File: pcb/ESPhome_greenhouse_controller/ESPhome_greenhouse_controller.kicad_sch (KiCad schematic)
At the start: 10 parts, among them K1 SANYOU_SRD_Form_C, K2 SANYOU_SRD_Form_C, K3 SANYOU_SRD_Form_C, K4 SANYOU_SRD_Form_C, K5 SANYOU_SRD_Form_C, K6 SANYOU_SRD_Form_C, U1 PC817, U2 PC817, U3 INA219AxD

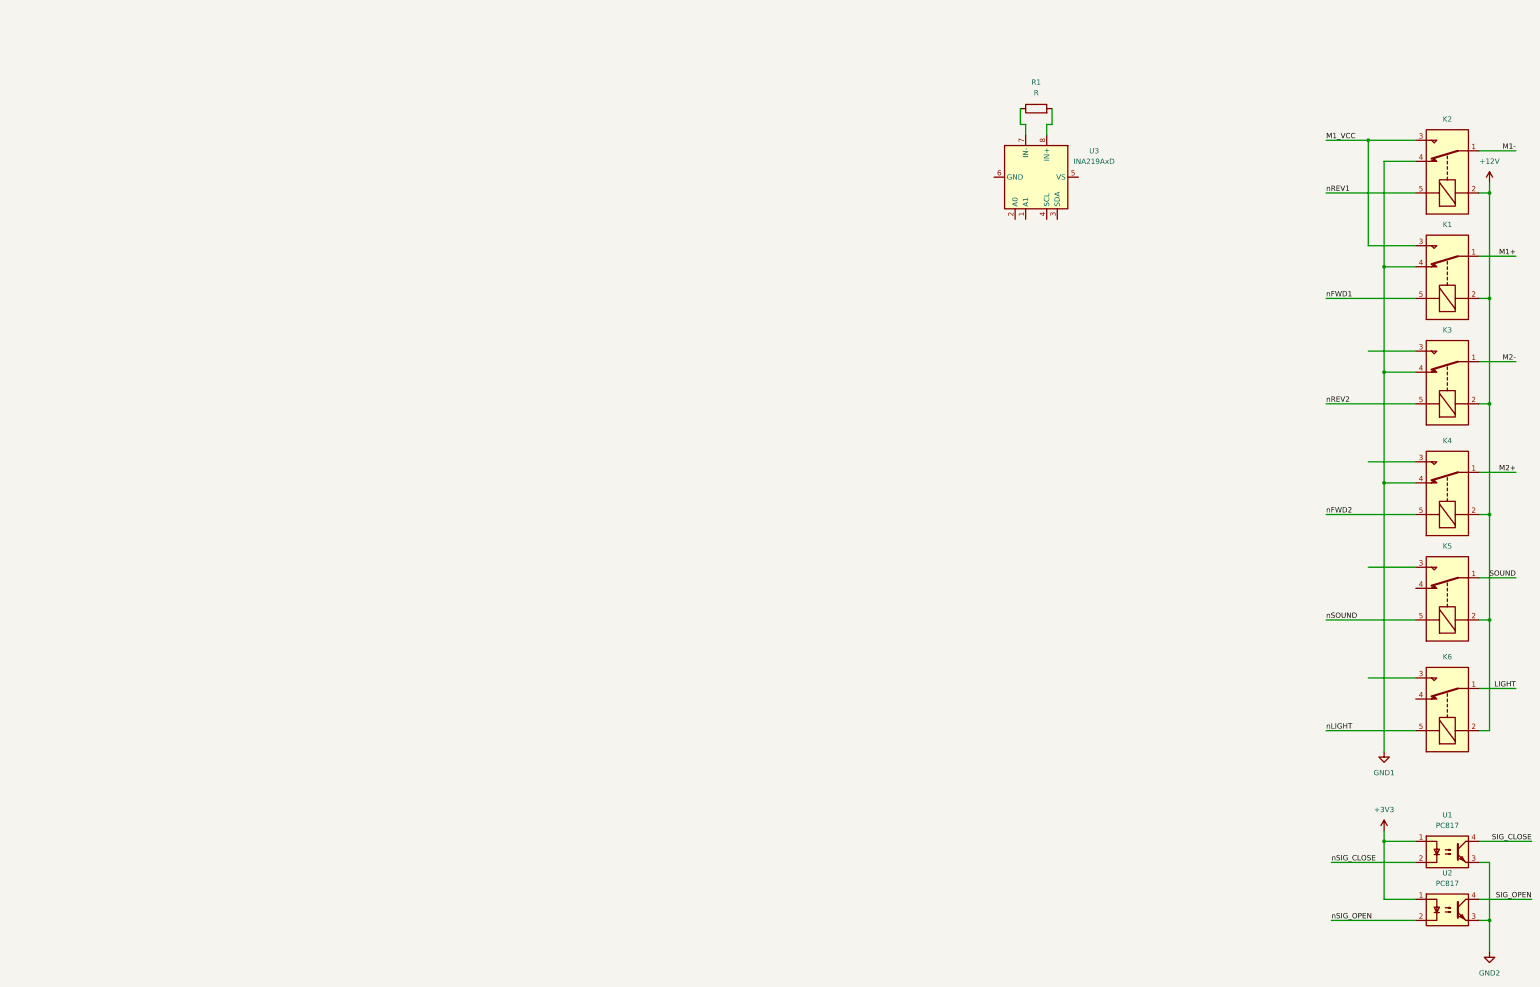
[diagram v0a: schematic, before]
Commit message: update
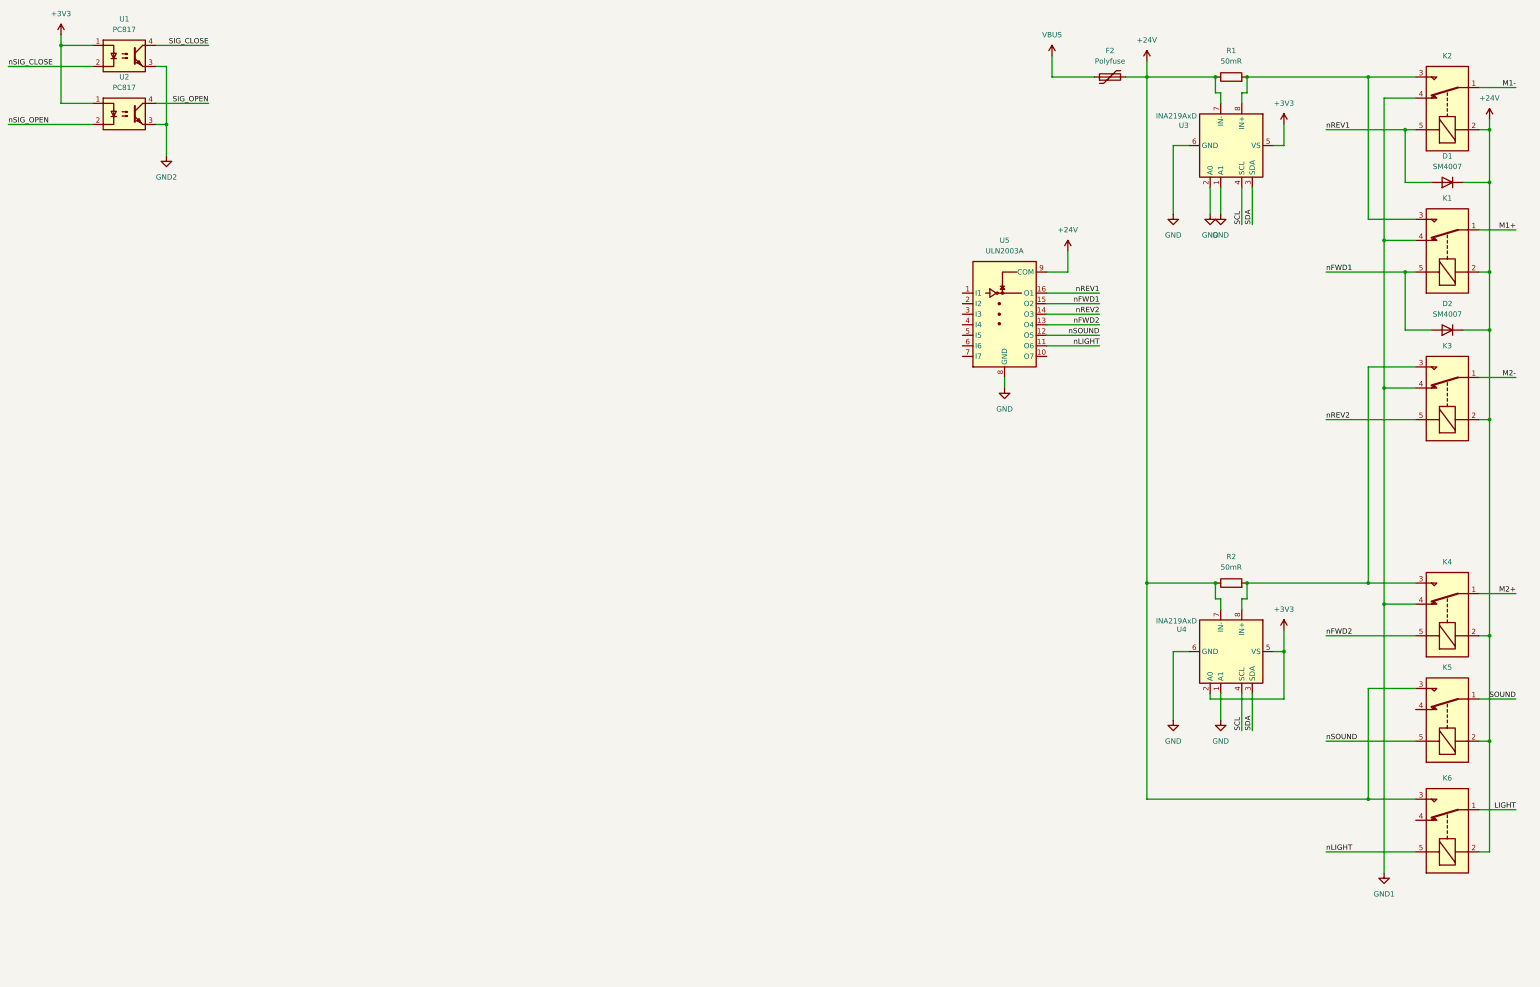
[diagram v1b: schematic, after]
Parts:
- added D1, D2: SM4007, Diode_SMD:D_MELF, symbol Diode:SM4007
- added F2: Polyfuse, Fuse:Fuse_Bourns_MF-RHT1100, symbol Device:Polyfuse
- added R2: 50mR, Resistor_SMD:R_1206_3216Metric, symbol Device:R
- added U4: INA219AxD, Package_SO:SOIC-8_3.9x4.9mm_P1.27mm, symbol Sensor_Energy:INA219AxD
- added U5: ULN2003A, symbol Transistor_Array:ULN2003A
- R1: value R -> 50mR; footprint (none) -> Resistor_SMD:R_1206_3216Metric
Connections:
- net +12V is gone; now on net +24V: K1.2, K2.2, K3.2, K4.2, K5.2, K6.2
- net M1_VCC is gone; now on an unnamed net: K1.3, K2.3
- net +3V3: now also U3.5 (VS), U4.2 (A0), U4.5 (VS)
- net nFWD1: now also D2.2 (A), U5.15 (O2)
- net nFWD2: now also U5.13 (O4)
- net nLIGHT: now also U5.11 (O6)
- net nREV1: now also D1.2 (A), U5.16 (O1)
- net nREV2: now also U5.14 (O3)
- net nSOUND: now also U5.12 (O5)
- net +24V: now reaches K5.3
- net +24V: now also K6.3, R1.1, U3.7 (IN-), D1.1 (K), D2.1 (K), F2.2, R2.1, U4.7 (IN-), U5.9 (COM)
- net at K4.3: now also K3.3, R2.2, U4.8 (IN+)
- net GND: now reaches U3.1 (A1)
- net GND: now also U3.2 (A0), U3.6 (GND), U4.1 (A1), U4.6 (GND), U5.8 (GND)
- net SDA: now reaches U3.3 (SDA)
- net SDA: now also U4.3 (SDA)
- net SCL: now reaches U3.4 (SCL)
- net SCL: now also U4.4 (SCL)
- new net VBUS: F2.1
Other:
- moved on the sheet: K1, K2, K3, K4, K5, K6, R1, U1, U2, U3
